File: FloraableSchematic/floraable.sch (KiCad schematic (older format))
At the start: 25 parts, among them J1 USB_B, J2 soil moisture sensor, J3 water pump, J4 LED strip, Q1 IRL1404Z, Q2 IRL1404Z, U1 MCP1702-3302E/TO, U2 BH1750_module, U3 NodeMCU, U4 DHT22

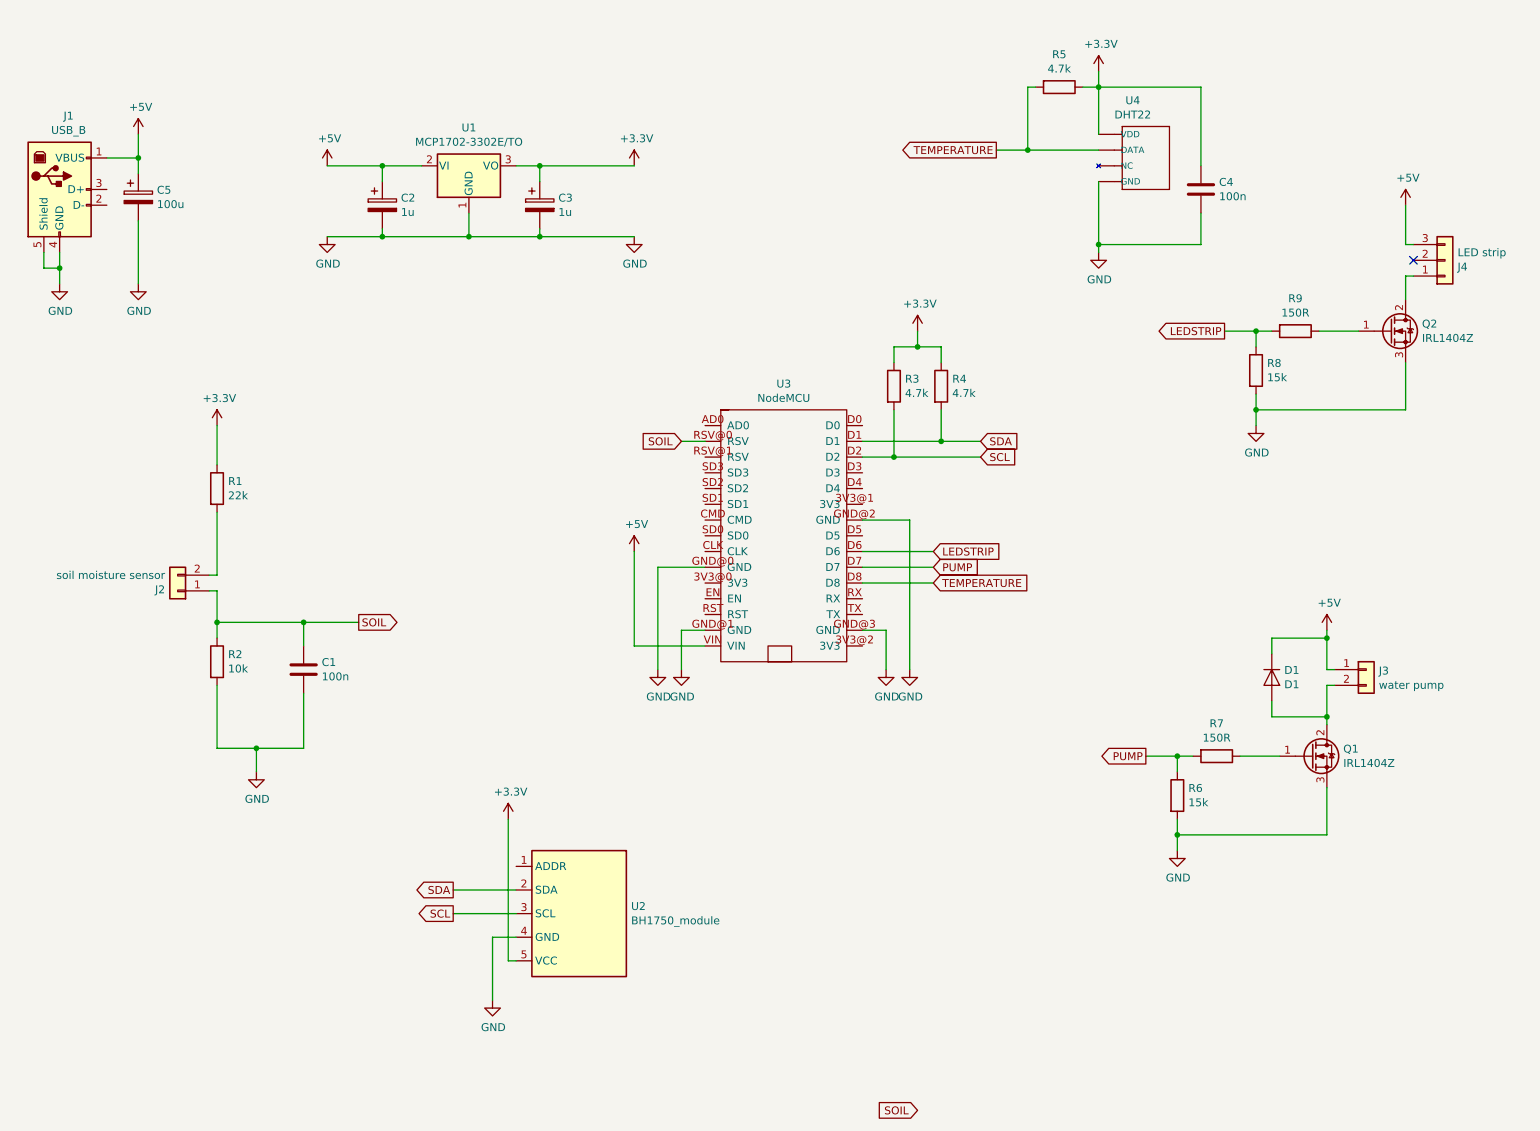
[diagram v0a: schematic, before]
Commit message: Add files via upload
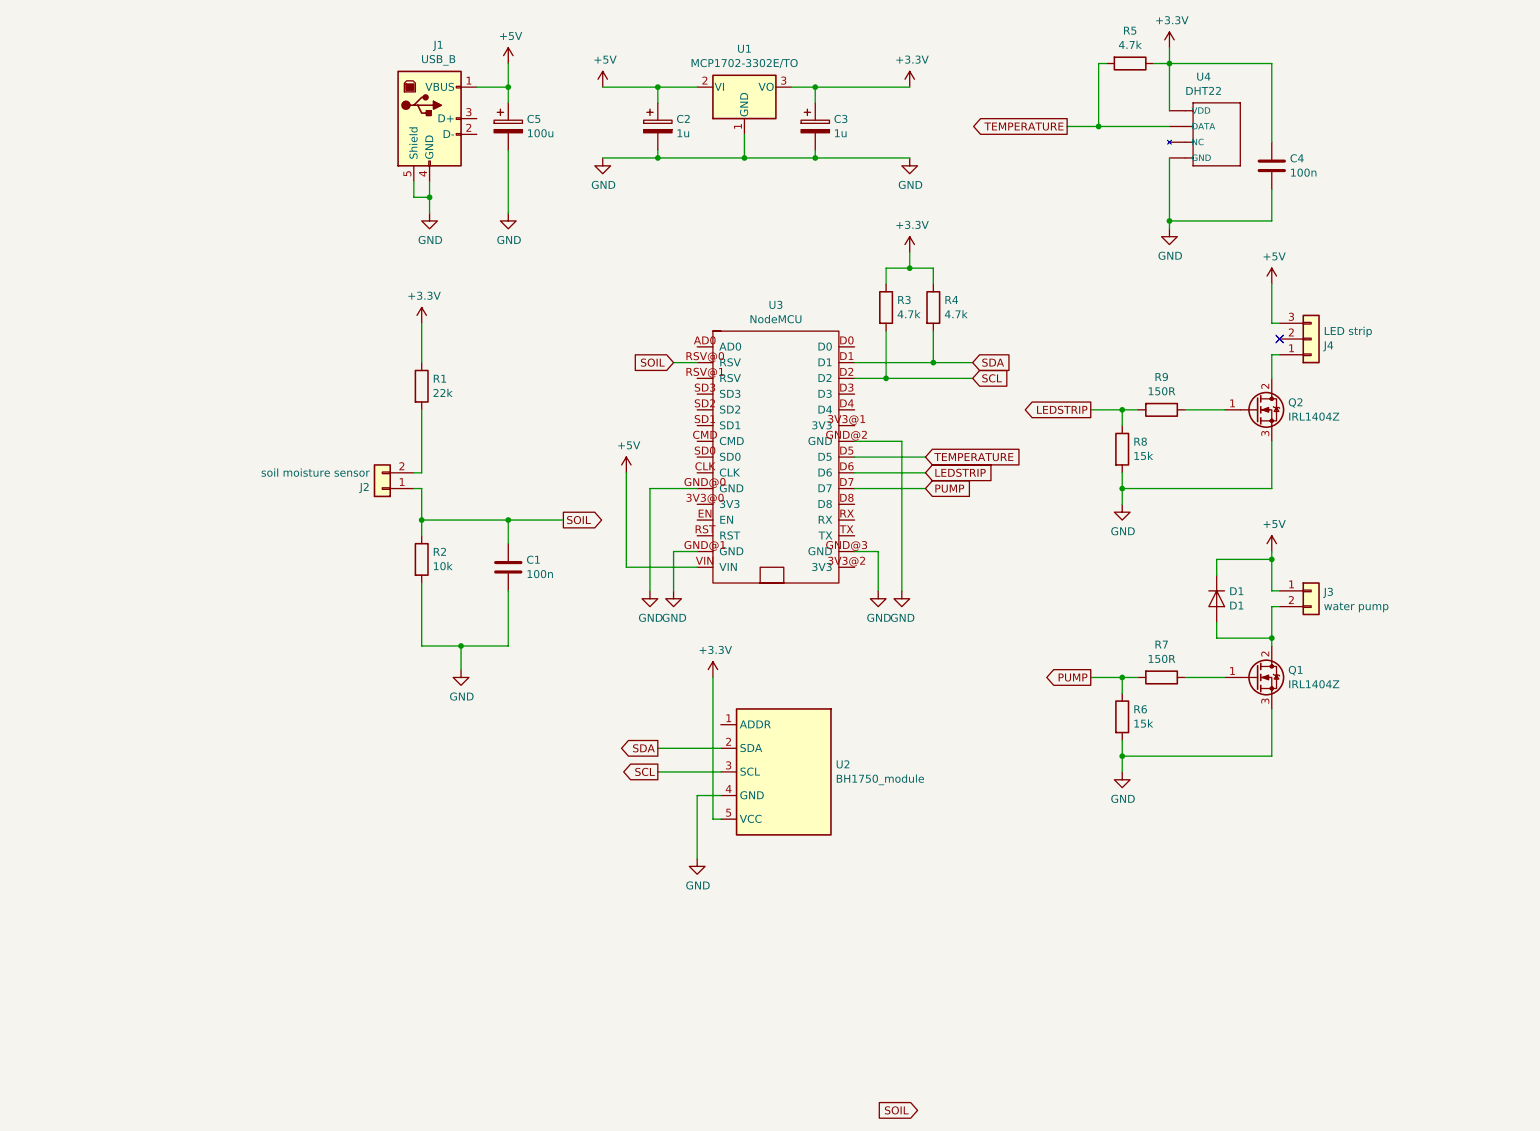
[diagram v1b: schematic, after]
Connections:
- net TEMPERATURE: now also U3.D5; no longer U3.D8
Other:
- moved on the sheet: C1, C2, C3, C4, C5, D1, J1, J2, J3, J4, Q1, Q2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
